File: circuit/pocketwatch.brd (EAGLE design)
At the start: 64.8 x 71.8 mm, 161 parts, among them M1 MOTOR, Q1 32.768 KHz, Q2 BUZZER, Q3 MOSFET, N CHANNEL, SOT23-3, U1 ATmega645PA, U2 MCP-LI-CHARGER-1, U3 TC54, X1 USB-MICRO_B

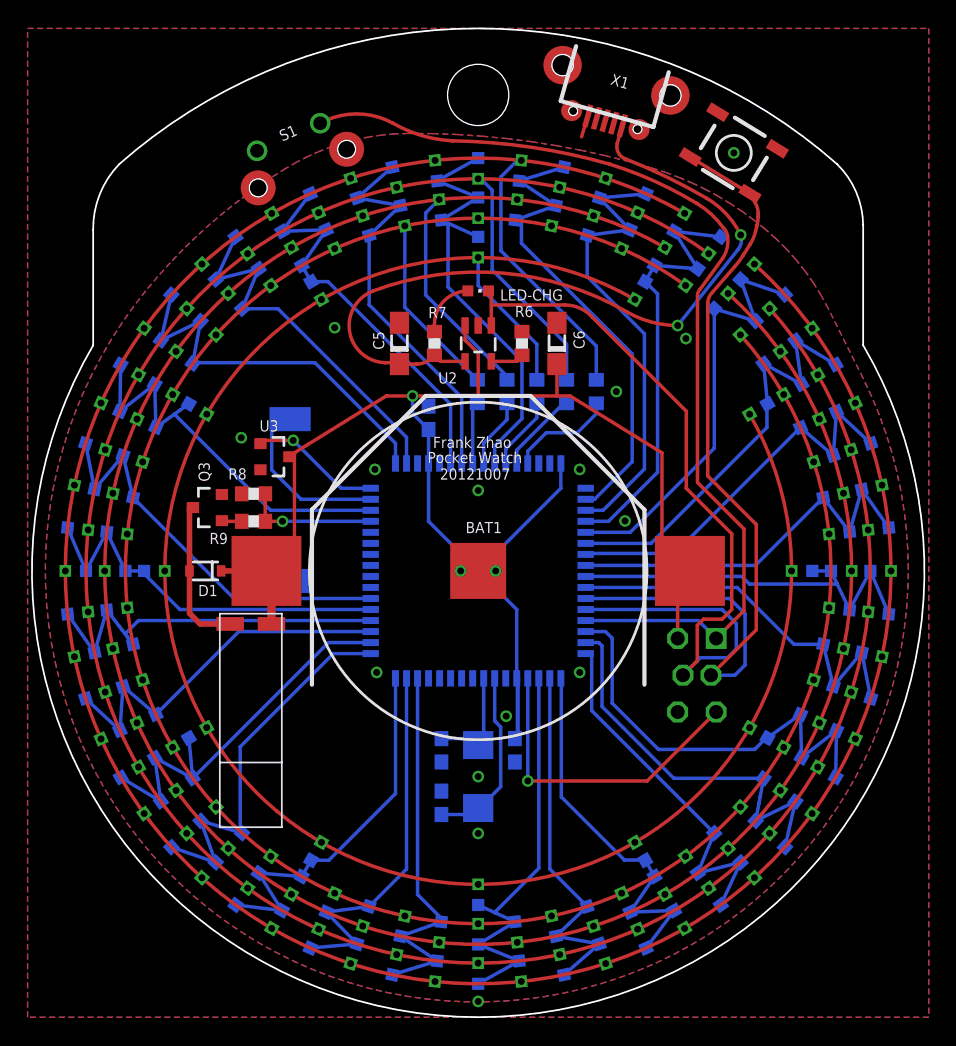
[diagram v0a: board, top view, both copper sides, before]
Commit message: circuit maintainance
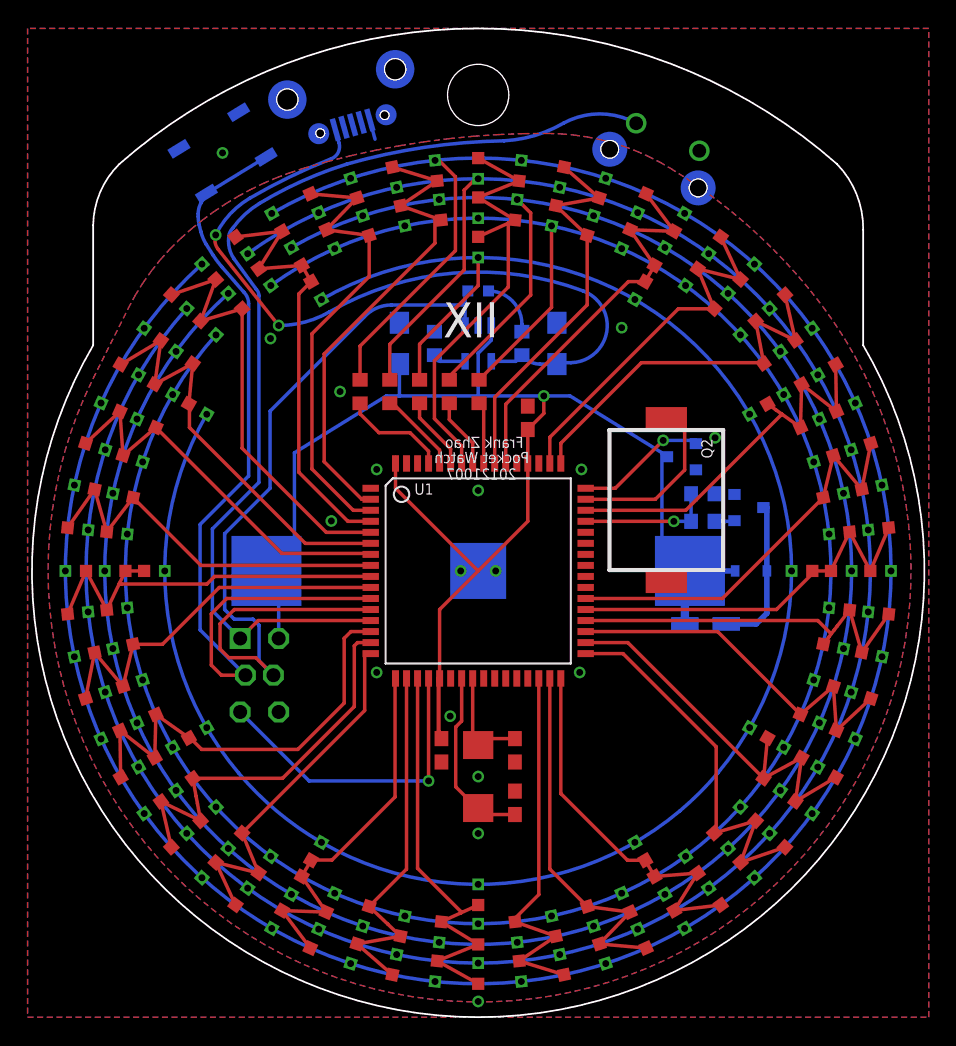
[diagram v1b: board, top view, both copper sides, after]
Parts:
- C1, C2, C3, C4: device rcl:C0603 -> pocketwatch:C0603
- C5, C6: device rcl:SMC_A -> pocketwatch:SMC_A
- R1, R2, R3, R4, R5, R6, R7, R8, R9: device rcl:R0603 -> pocketwatch:R0603
- moved LED16 58.4 mm to (29.2, 0.00), flipped to the top
- moved LED46 58.4 mm to (-29.2, 0.00), flipped to the top
- moved LED15 58.1 mm to (29.1, 3.05), flipped to the top
- moved LED17 58.1 mm to (29.1, -3.05), flipped to the top
- moved LED45 58.1 mm to (-29.1, -3.05), flipped to the top
- moved LED47 58.1 mm to (-29.1, 3.05), flipped to the top
- moved LED14 57.1 mm to (28.6, 6.07), flipped to the top
- moved LED18 57.1 mm to (28.6, -6.07), flipped to the top
- moved LED44 57.1 mm to (-28.6, -6.07), flipped to the top
- moved LED48 57.1 mm to (-28.6, 6.07), flipped to the top
- moved LED13 55.6 mm to (27.8, 9.03), flipped to the top
- moved LED19 55.6 mm to (27.8, -9.03), flipped to the top
- moved LED43 55.6 mm to (-27.8, -9.03), flipped to the top
- moved LED49 55.6 mm to (-27.8, 9.03), flipped to the top
- moved LED12 53.4 mm to (26.7, 11.9), flipped to the top
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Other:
- outline, holes or cut-outs redrawn
